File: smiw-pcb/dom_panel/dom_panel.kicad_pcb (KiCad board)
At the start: 2 copper layers, 7 parts, among them J1 4-1734839-5, J2 Barrel_Jack_Switch, U1 ESP32-S3-DEVKITC-1-N8R8, U2 SN74AVC16T245DGGR, U3 SN74AVC16T245DGGR, U4 PT4115, U5 REG1117A

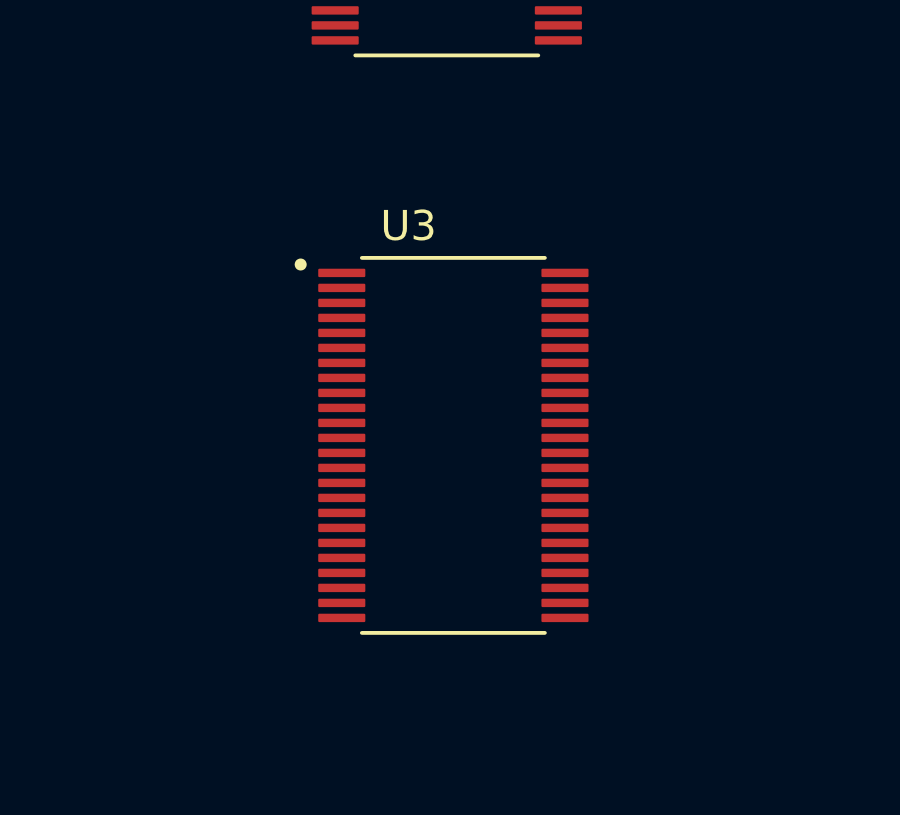
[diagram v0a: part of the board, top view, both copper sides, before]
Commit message: wsszystko
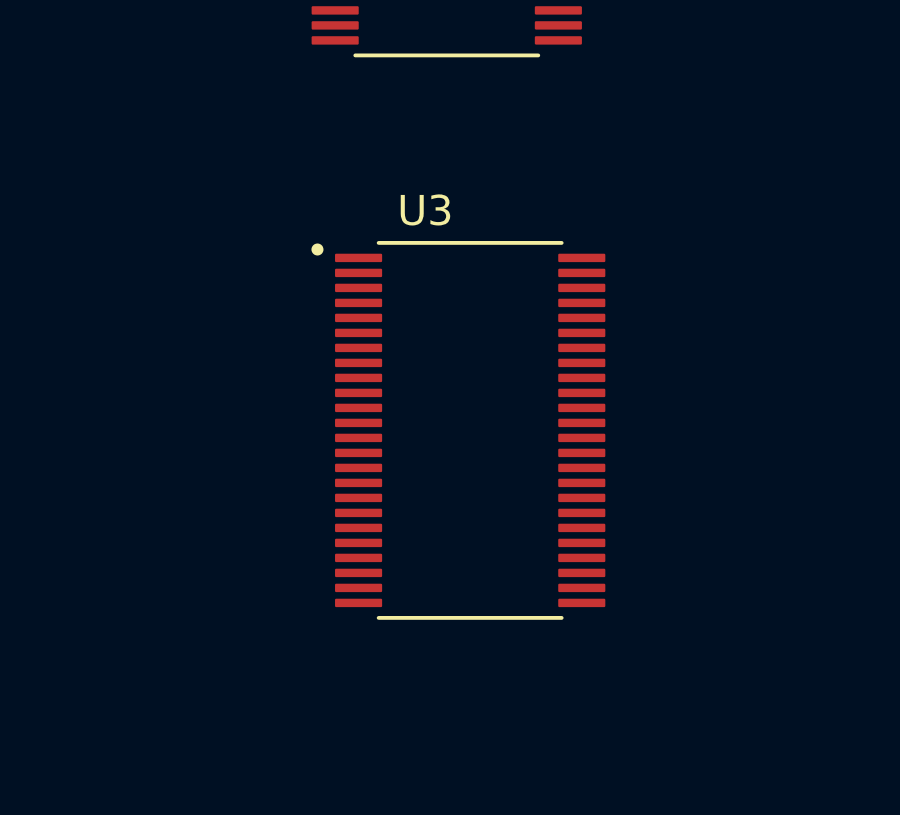
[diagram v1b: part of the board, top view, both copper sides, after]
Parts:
- moved U3 0.75 mm to (146.3, 96.2)
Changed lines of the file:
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@@
 	(footprint "SN74AVC16T245DGGR:SOP50P810X120-48N"
 		(layer "F.Cu")
-		(at 145.72 96.75)
+		(at 146.28 96.25)
 		(property "Reference" "U3"
 			(at -1.495 -7.312 0)
